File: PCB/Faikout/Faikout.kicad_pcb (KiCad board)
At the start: 2 copper layers, 70 x 70 mm, 47 parts, among them J1 1x5, J2 TC2030-USB-NL, J3 Reset, Q1 BSS138PS, U1 TPS562246, U4 ESP32-S3-MINI-1-N4R2

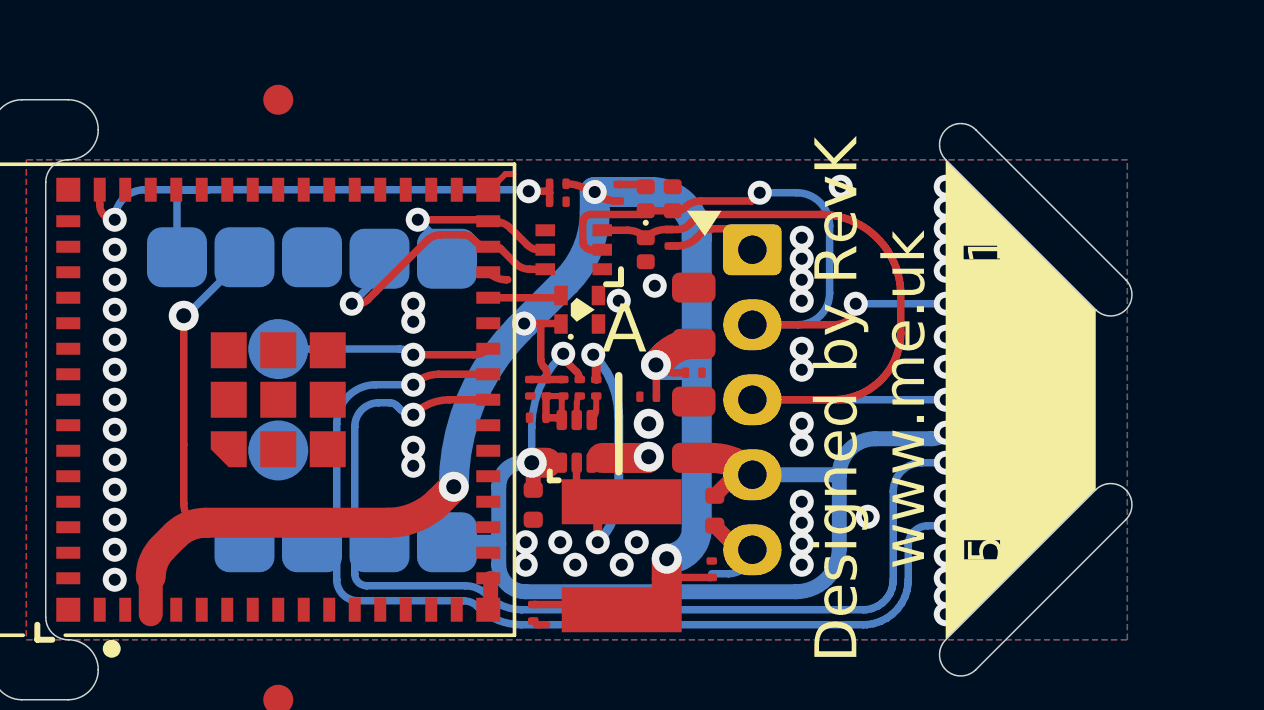
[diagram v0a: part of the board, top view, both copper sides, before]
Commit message: Tidy for order
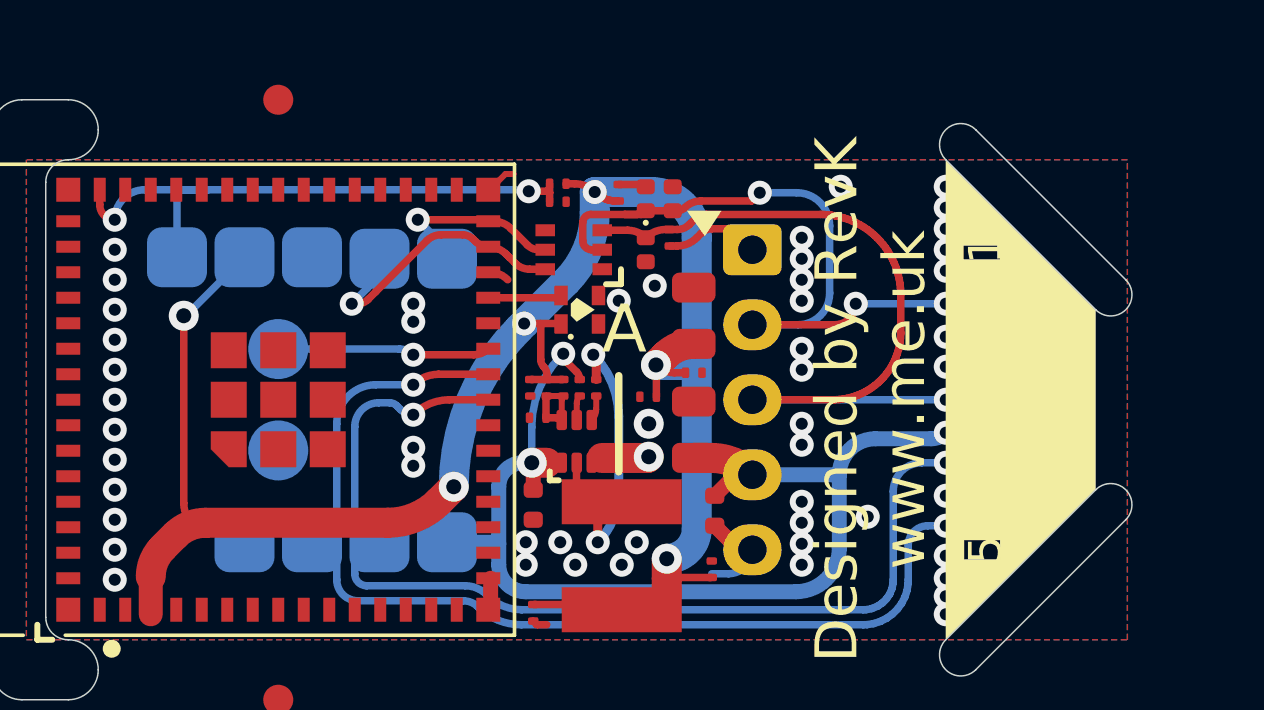
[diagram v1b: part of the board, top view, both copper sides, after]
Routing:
- net Net-(D4-K): track 33.7 -> 34.6 mm
